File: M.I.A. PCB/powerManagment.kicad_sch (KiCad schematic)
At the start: 41 parts, among them J3 Screw_Terminal_01x02, J4 Screw_Terminal_01x02, J5 Conn_01x02_Pin, U10 INA219AxDCN, U11 AP2112K-3.3, U12 AP62150WU, U13 TPS2121RUXR, U14 AP62150WU, U9 TPS2121RUXR

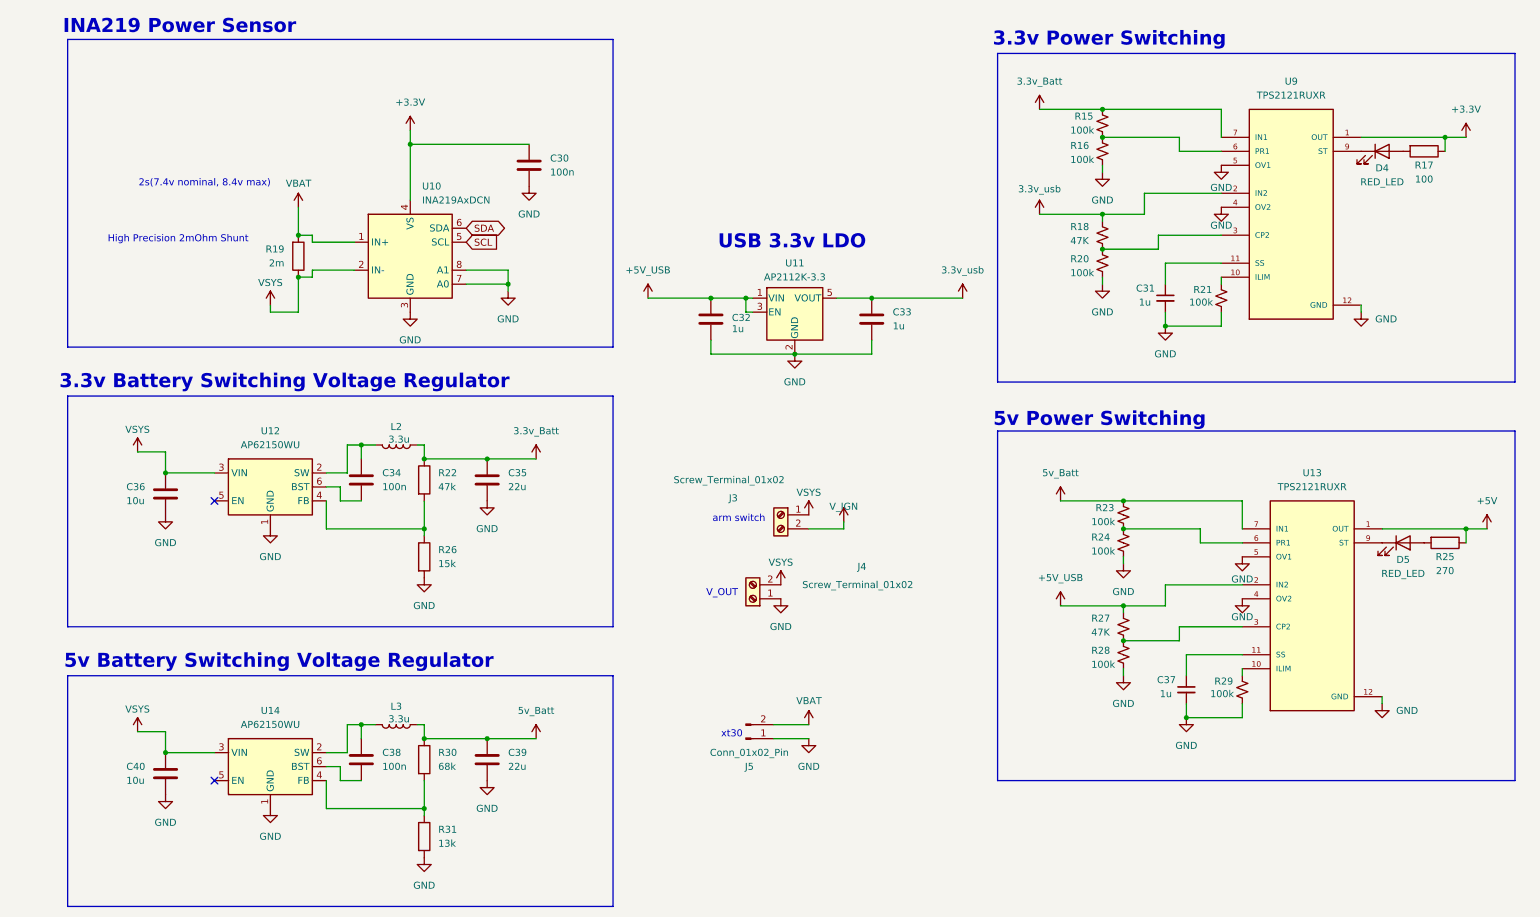
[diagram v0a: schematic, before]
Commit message: More Small Updates/Improvements
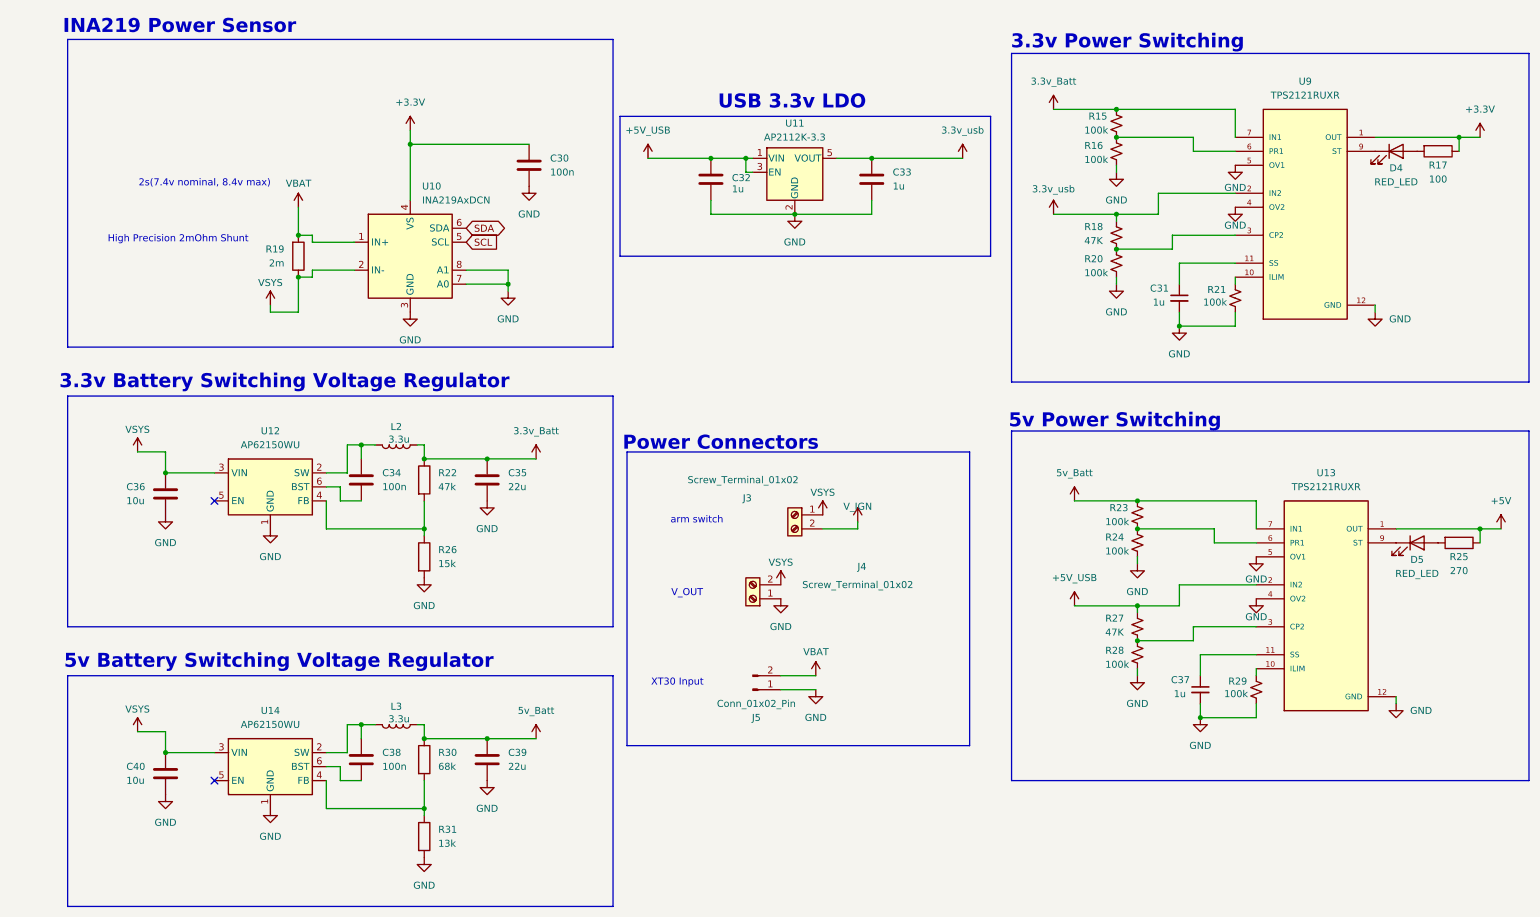
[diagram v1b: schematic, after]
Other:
- note added: "Power Connectors"
- note added: "XT30 Input"
- note removed: "xt30"
- moved on the sheet: C31, C32, C33, C37, D4, D5, J3, J5, R15, R16, R17, R18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
